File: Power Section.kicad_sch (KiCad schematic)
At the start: 55 parts, among them CN1 S2B-PH-SM4-TB, J1 USB_C_Receptacle_USB2.0, Q2 SSM3J328R,LF, U15 TPS63031DSK, U16 LPS3015-152MRC, U17 MAX17048, U5 MP2617AGL-Z, U6 USBLC6-2SC6

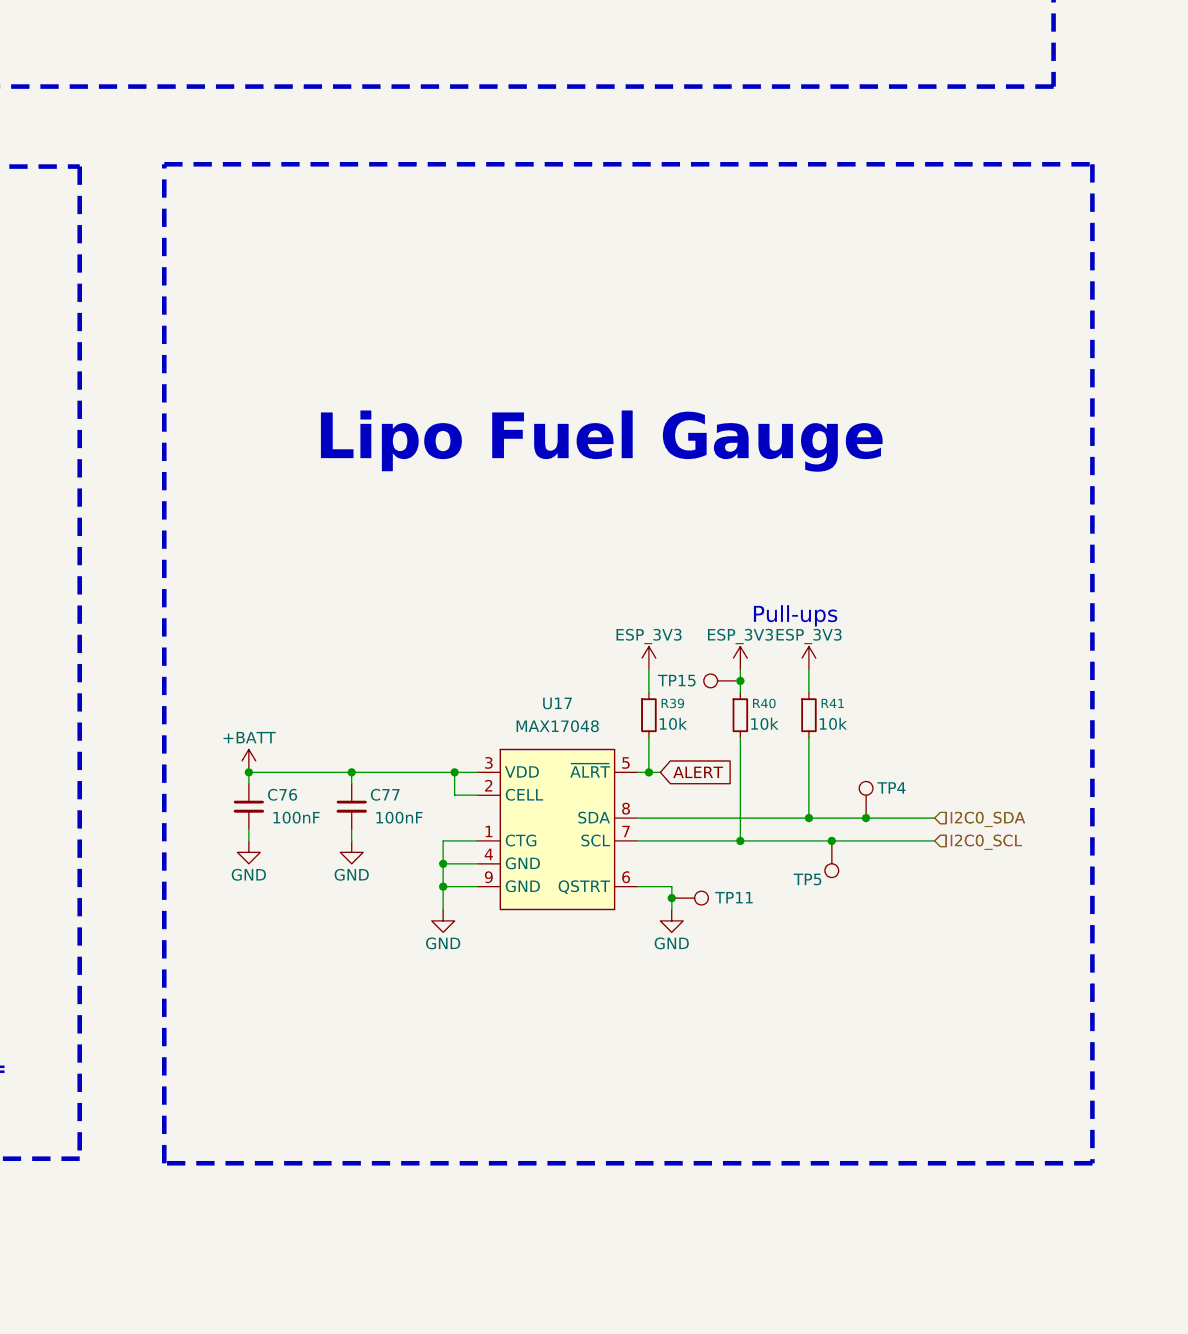
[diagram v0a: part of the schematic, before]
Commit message: Did the layout plan
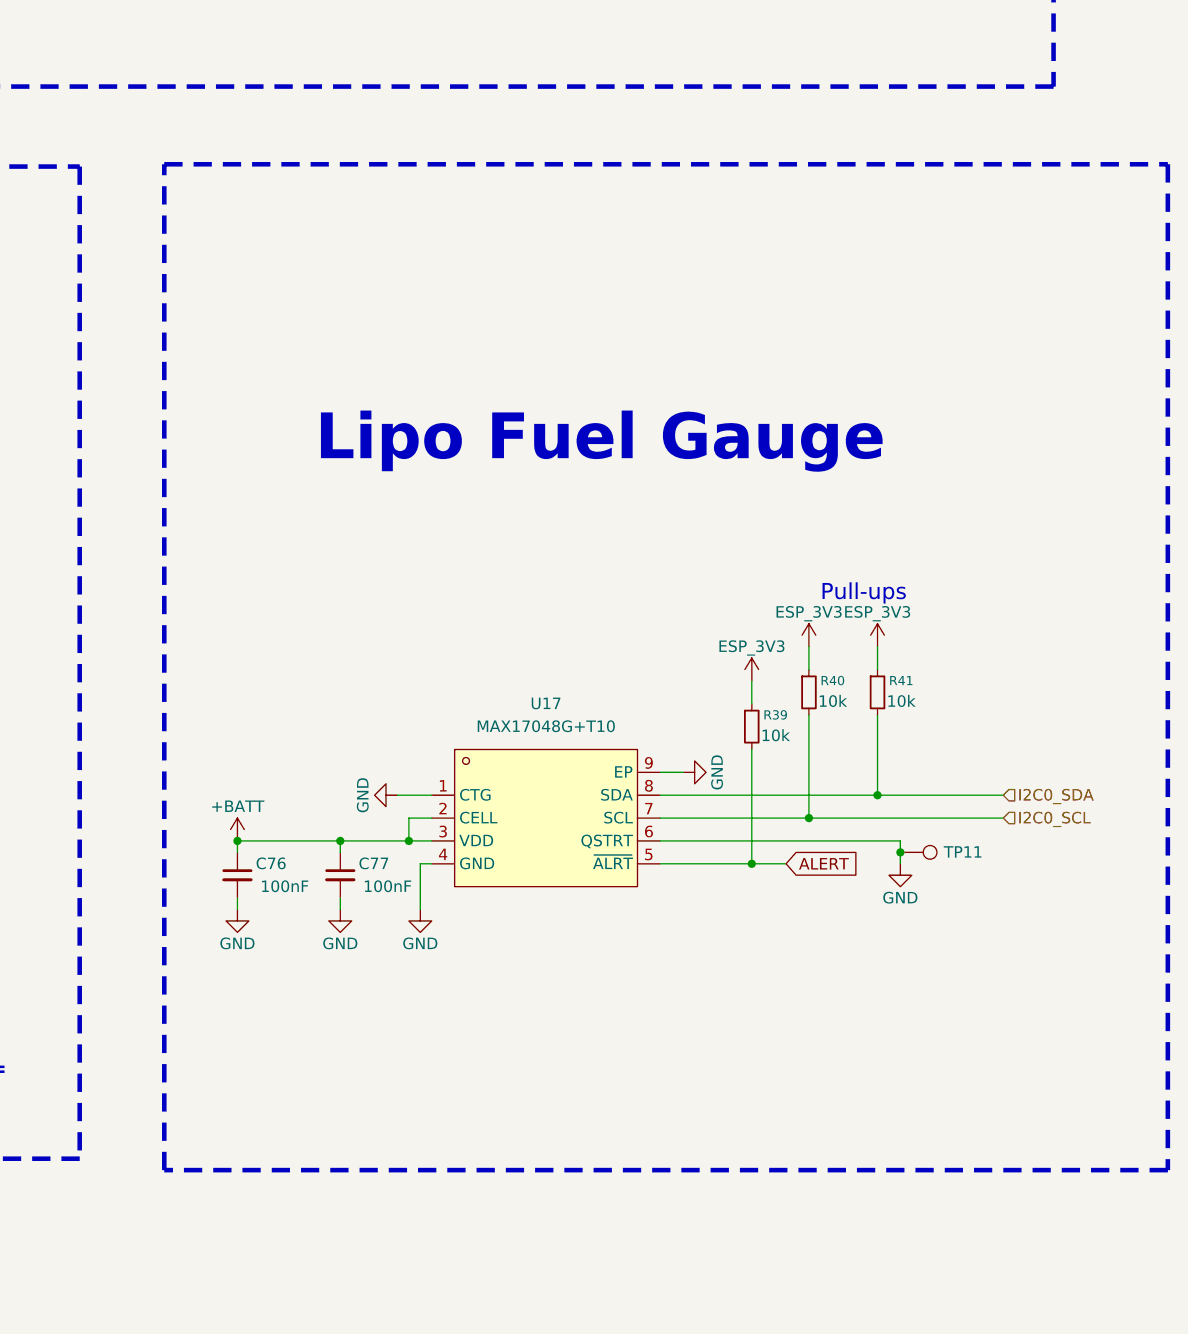
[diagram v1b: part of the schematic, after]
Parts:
- removed TP15, TP4, TP5: TestPoint, TestPoint:TestPoint_Pad_D1.5mm, symbol Connector:TestPoint
- removed U17: MAX17048, Abhishek_Library:SON50P200X200X80-9N, symbol PCM_marbastlib-various:MAX17048
- added U17: MAX17048G+T10, MAX17048:TDFN-8_L2.0-W2.0-P0.50-BL-EP1.2, symbol MAX17048:MAX17048G+T10
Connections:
- net +BATT: now also U17.2 (CELL), U17.3 (VDD)
- net ALERT: now also U17.5 (~{ALRT})
- net GND: now also U17.1 (CTG), U17.4 (GND), U17.6 (QSTRT), U17.9 (EP)
- net I2C0_SCL: now also U17.7 (SCL)
- net I2C0_SDA: now also U17.8 (SDA)
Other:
- moved on the sheet: C76, C77, R39, R40, R41, TP11

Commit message: Done with the routing. Yet to correct the issue raised and review the whole design
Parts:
- C16, C75, C84: LCSC (none) -> C14663
- C18, C85: LCSC (none) -> C15849
- R35, R36, R38: LCSC (none) -> C49330116
- R39, R40, R41: LCSC C177644 -> C49330116
- R49: LCSC (none) -> C25803
- U15: LCSC Part (none) -> C15516
